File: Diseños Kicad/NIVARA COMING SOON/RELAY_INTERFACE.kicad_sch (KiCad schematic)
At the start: 3 parts, among them K1 G2RL-1, K2 G2RL-1

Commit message: a
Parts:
- U4: footprint Riqi_Parts:SOIC127P600X172-14N -> Package_TO_SOT_SMD:Infineon_PG-TO-220-7Lead_TabPin8
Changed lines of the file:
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@@
 			)
 		)
-		(property "Footprint" "Riqi_Parts:SOIC127P600X172-14N"
+		(property "Footprint" "Package_TO_SOT_SMD:Infineon_PG-TO-220-7Lead_TabPin8"
 			(at 88.9 59.69 0)
 			(effects

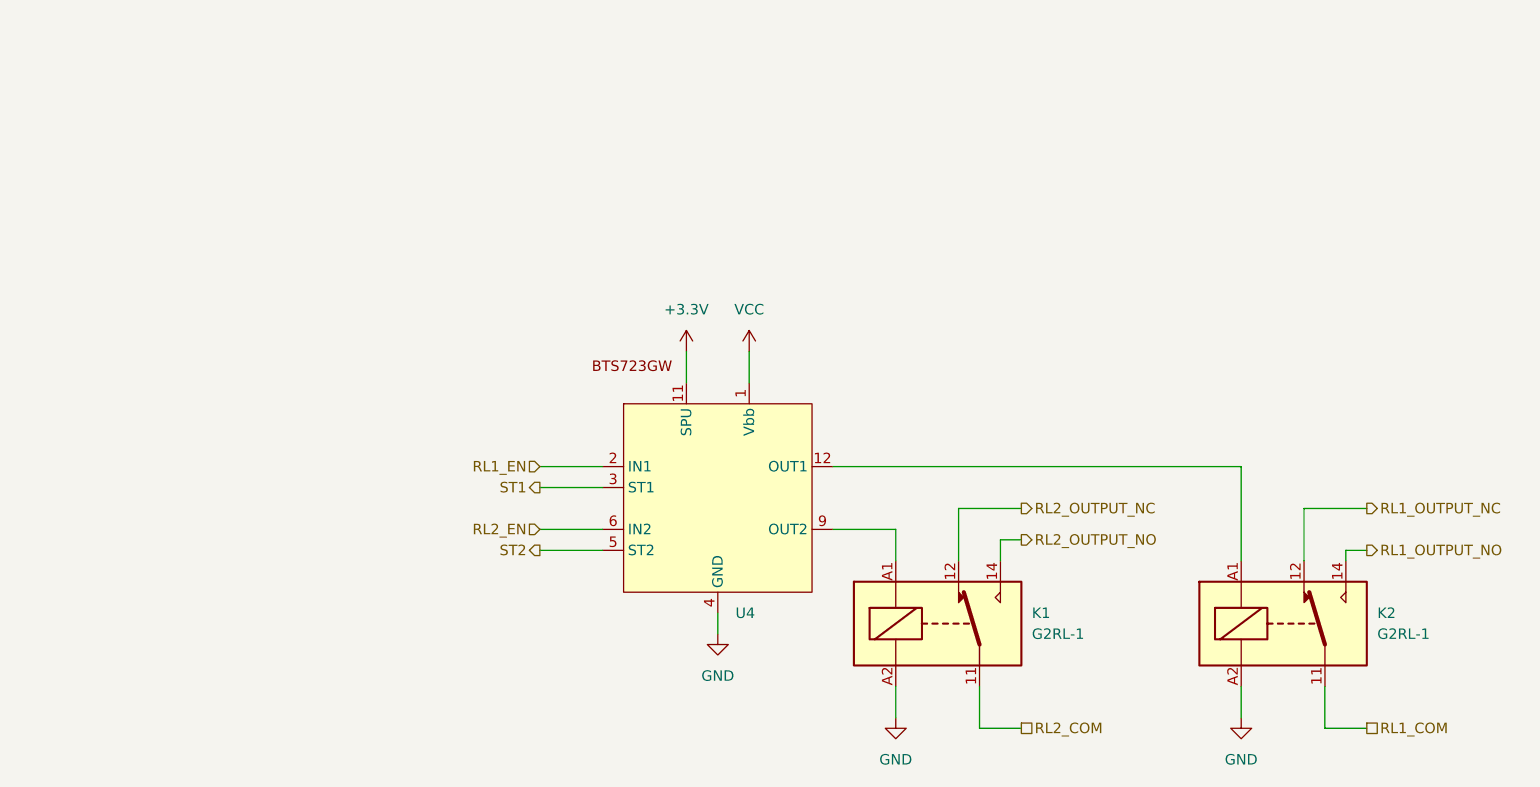
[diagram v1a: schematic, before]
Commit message: AMEN
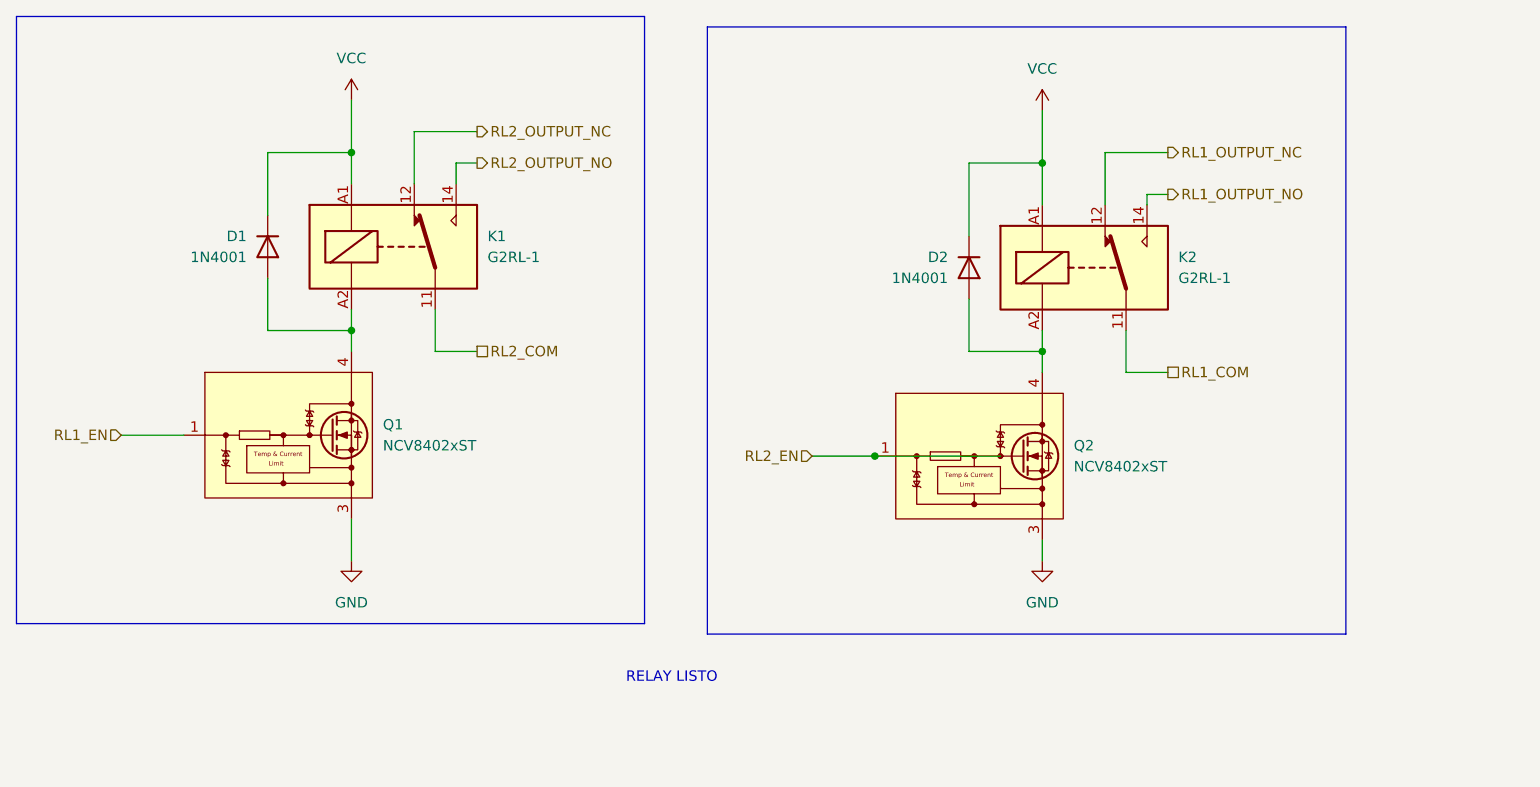
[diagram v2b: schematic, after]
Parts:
- removed U4: ~, Package_TO_SOT_SMD:Infineon_PG-TO-220-7Lead_TabPin8, symbol Riqi_Parts:BTS723GW
- added D1, D2: 1N4001, Diode_SMD:D_SMA, symbol Diode:1N4001
- added Q1, Q2: NCV8402xST, Package_TO_SOT_SMD:SOT-223, symbol Driver_FET:NCV8402xST
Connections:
- net GND: now also Q1.3 (S), Q2.3 (S); no longer K1.A2, K2.A2
- net RL1_EN: now also Q1.1 (G)
- net RL2_EN: now also Q2.1 (G)
- net VCC: now also K1.A1, K2.A1, D1.1 (K), D2.1 (K)
- new net: D1.2 (A), K1.A2, Q1.2 (D), Q1.4 (D)
- new net: D2.2 (A), K2.A2, Q2.2 (D), Q2.4 (D)
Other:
- note added: "RELAY LISTO"
- moved on the sheet: K1, K2
